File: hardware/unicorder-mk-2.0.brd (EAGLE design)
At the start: 38.2 x 32.3 mm, 13 parts, among them IC1 TINY85

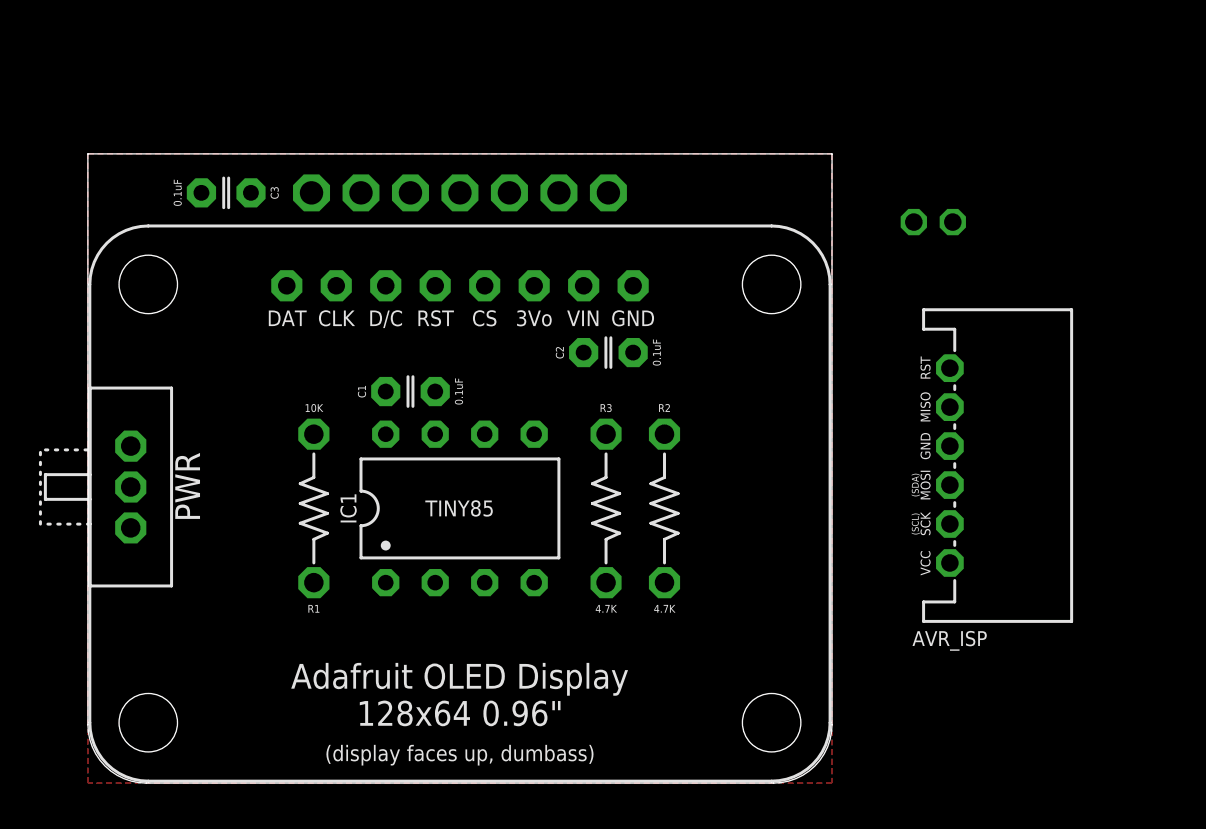
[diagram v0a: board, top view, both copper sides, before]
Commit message: alsdkfjkalsdf
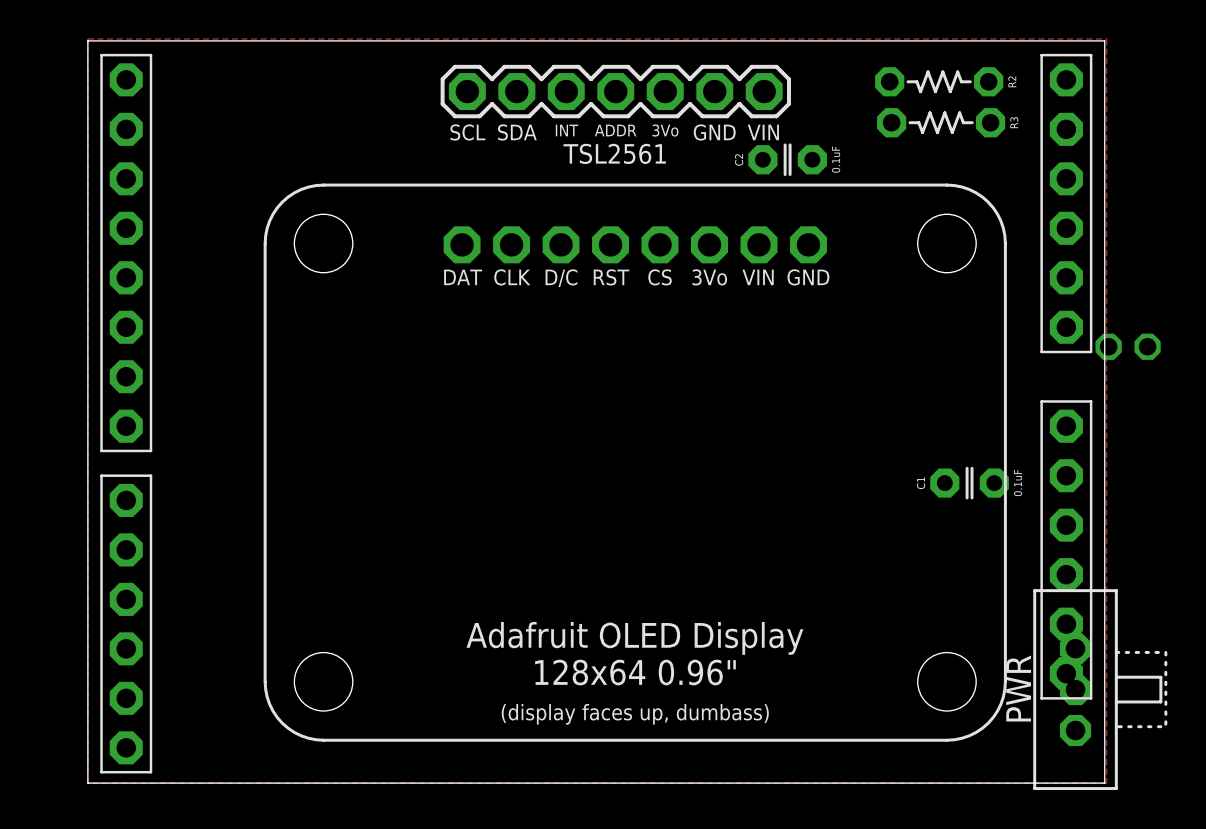
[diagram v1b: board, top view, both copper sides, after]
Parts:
- removed AVR_ISP: AVR_SPI_PRG_6AVR-JST-PTH-RA-I2C, A_butts:AVR-JST-6-PTH-RA-I2C
- removed C3: 0.1uF, A_butts:C025-024X044
- removed IC1: TINY85, A_butts:DIP08
- removed R1: 10K, A_butts:RESISTOR-AXIAL-PTH-7.62MM
- added SHIELD: (no value), A_butts:ARDUINO_SHIELD_NOOUTLINE_INSIDE_SMALLER
- DISPLAY1: value ADAFRUIT_128X64_OLED -> ADAFRUIT_128X64_OLEDCLOSER; device A_butts:ADAFRUIT_128X64_OLED -> A_butts:ADAFRUIT_128X64_OLED_CLOSER
- R2, R3: device A_butts:RESISTOR-AXIAL-PTH-7.62MM -> A_butts:RESISTOR-AXIAL-PTH-5.08MM
- moved PWR 49.6 mm to (50.6, 4.80), turned to 90 degrees
- moved C1 29.1 mm to (45.2, 15.4)
- moved R3 26.2 mm to (43.7, 33.9), turned to 180 degrees
- moved R2 26.0 mm to (43.6, 36.0), turned to 180 degrees
- moved C2 13.5 mm to (35.8, 32.0)
- moved BATT 11.9 mm to (53.3, 22.4)
- moved DISPLAY1 9.24 mm to (28.0, 27.6)
- moved TSL2561 8.91 mm to (19.4, 35.5), flipped to the top
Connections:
- removed net MISO: AVR_ISP.MISO, IC1.6
- removed net RST: AVR_ISP.RESET, IC1.1, R1.P$1
- net DISPLAY_RST: no longer IC1.2
- net GND: no longer AVR_ISP.GND, C3.2, IC1.4
- net MOSI/SDA: no longer AVR_ISP.MOSI/SDA, IC1.5
- net SCK/SCL: no longer AVR_ISP.SCK, IC1.7
- net VCC: no longer AVR_ISP.VCC, C3.1, IC1.8, R1.P$2
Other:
- board size 38.2 x 32.3 mm -> 52.2 x 38.1 mm
